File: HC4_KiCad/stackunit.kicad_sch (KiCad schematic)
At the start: 18 parts, among them IC11 74HC161, IC12 74HC377

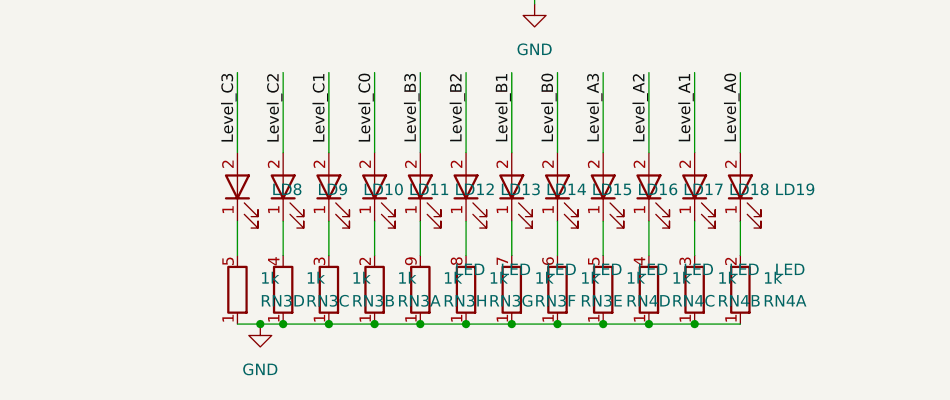
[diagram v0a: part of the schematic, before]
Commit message: 基板ぬ
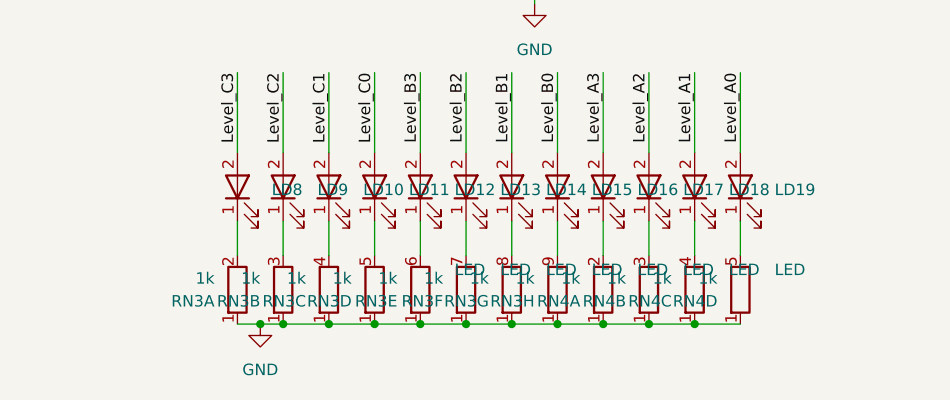
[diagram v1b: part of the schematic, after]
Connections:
- net at LD10.1 (K): now also RN3.4 (R3.2); no longer RN3.3 (R2.2)
- net at RN4.2 (R1.2): now also LD16.1 (K); no longer LD19.1 (K)
- net at RN4.3 (R2.2): now also LD17.1 (K); no longer LD18.1 (K)
- net at RN3.5 (R4.2): now also LD11.1 (K); no longer LD8.1 (K)
- net at RN3.9 (R8.2): now also LD15.1 (K); no longer LD12.1 (K)
- net at RN3.2 (R1.2): now also LD8.1 (K); no longer LD11.1 (K)
- net at RN4.4 (R3.2): now also LD18.1 (K); no longer LD17.1 (K)
- net at RN3.6 (R5.2): now also LD12.1 (K); no longer LD15.1 (K)
- net at RN4.5 (R4.2): now also LD19.1 (K); no longer LD16.1 (K)
- net at LD14.1 (K): now also RN3.8 (R7.2); no longer RN3.7 (R6.2)
- net at LD9.1 (K): now also RN3.3 (R2.2); no longer RN3.4 (R3.2)
- net at LD13.1 (K): now also RN3.7 (R6.2); no longer RN3.8 (R7.2)
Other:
- moved on the sheet: RN3A, RN3B, RN3C, RN3D, RN3E, RN3F, RN3G, RN3H, RN4A, RN4B, RN4C, RN4D
